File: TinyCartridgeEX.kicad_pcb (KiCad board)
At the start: 2 copper layers, 62 x 81.1 mm, 27 parts, among them J1 Conn_01x24, J2 Conn_01x24, U1 SN74LVC8T245, U2 SN74LVC8T245, U3 SN74LVC8T245, U4 74LV17A, U5 74LVC06A, U6 74LVC1G06, U7 74LVC2G132, U9 TinyFPGA_EX, X1 EXPANSION_PORT_C64_EDGE

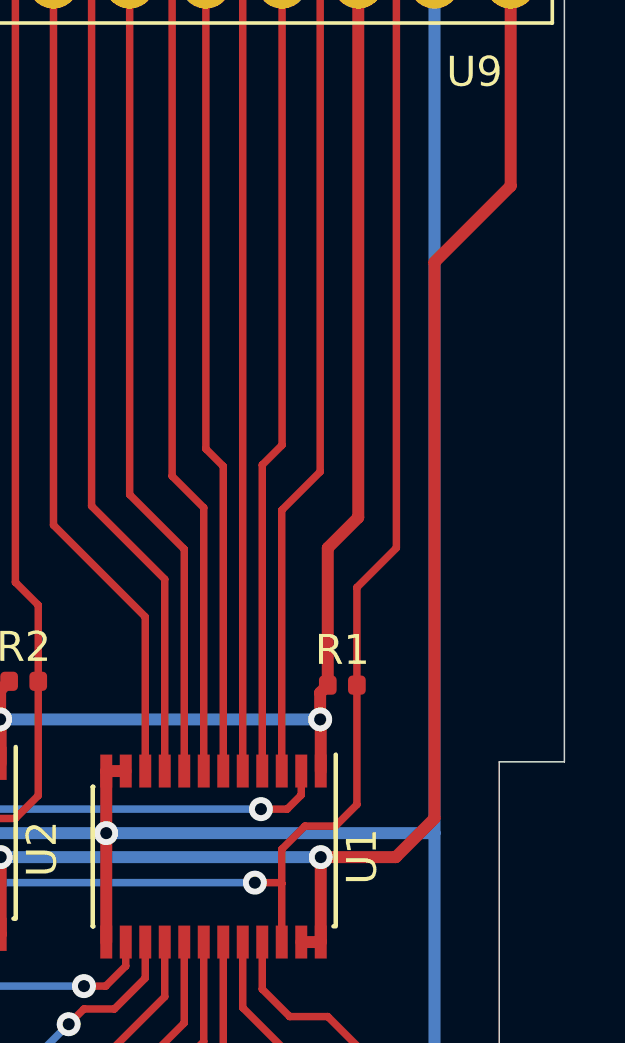
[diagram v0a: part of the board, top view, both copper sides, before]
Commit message: Add diode to Vin
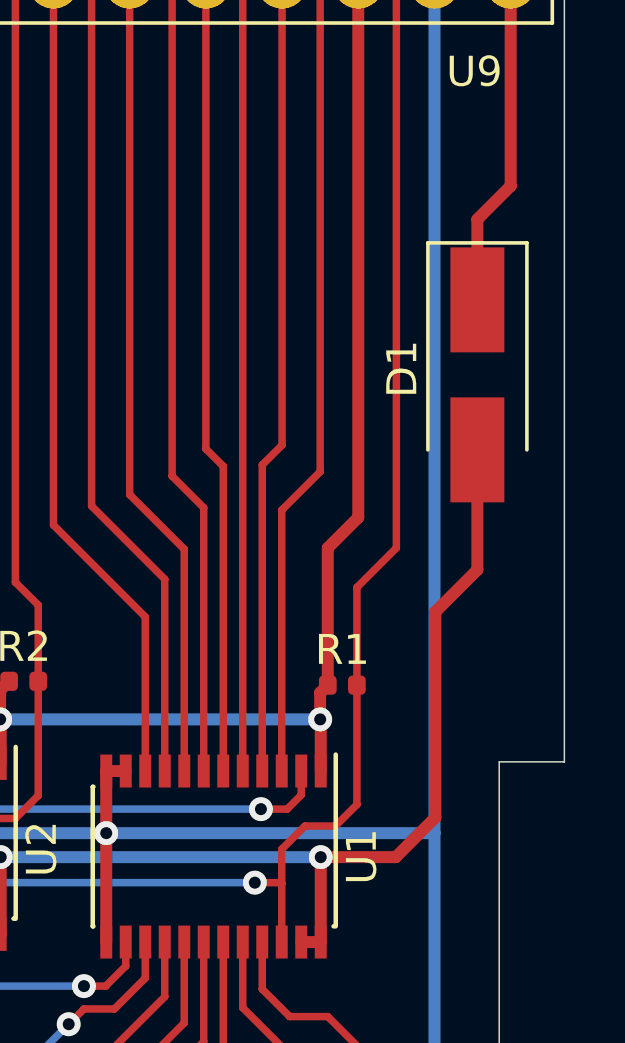
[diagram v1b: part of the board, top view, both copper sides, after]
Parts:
- added D1: EC30QSA045, Diode_SMD:D_SMA_Handsoldering, F.Cu at (104.3, 127.2)
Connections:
- U9 pad 48: +5V -> Net-(D1-Pad1)
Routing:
- net +5V: track 123.3 -> 107.2 mm
- net Net-(D1-Pad1): track 0.00 -> 11.0 mm
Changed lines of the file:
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@@
     (thickness 1.6)
     (drawings 20)
-    (tracks 723)
+    (tracks 726)
     (zones 0)
-    (modules 27)
-    (nets 85)
+    (modules 28)
+    (nets 86)
   )
   (page A4)
@@
   (net 83 "Net-(U7-Pad2)")
   (net 84 "Net-(U7-Pad1)")
+  (net 85 "Net-(D1-Pad1)")
   (net_class Default "This is the default net class."
     (clearance 0.2)
@@
     (add_net +5V)
     (add_net GND)
+    (add_net "Net-(D1-Pad1)")
     (add_net VCC)
+  )
+  (module Diode_SMD:D_SMA_Handsoldering (layer F.Cu)
+    (at 104.3 127.2 270)
+    (descr "Diode SMA (DO-214AC) Handsoldering")
+    (tags "Diode SMA (DO-214AC) Handsoldering")
+    (attr smd)
+    (fp_text reference D1 (at -0.2 2.5 90) (layer F.SilkS)
+      (effects (font (size 1 1) (thickness 0.15)))
+    )
+    (fp_text value EC30QSA045 (at 0 2.6 90) (layer F.Fab)
+      (effects (font (size 1 1) (thickness 0.15)))
+    )
+    (fp_line (start -4.4 -1.65) (end 2.5 -1.65) (layer F.SilkS) (width 0.12))
+    (fp_line (start -4.4 1.65) (end 2.5 1.65) (layer F.SilkS) (width 0.12))
+    (fp_line (start -0.64944 0.00102) (end 0.50118 -0.79908) (layer F.Fab) (width 0.1))
+    (fp_line (start -0.64944 0.00102) (end 0.50118 0.75032) (layer F.Fab) (width 0.1))
+    (fp_line (start 0.50118 0.75032) (end 0.50118 -0.79908) (layer F.Fab) (width 0.1))
+    (fp_line (start -0.64944 -0.79908) (end -0.64944 0.80112) (layer F.Fab) (width 0.1))
+    (fp_line (start 0.50118 0.00102) (end 1.4994 0.00102) (layer F.Fab) (width 0.1))
+    (fp_line (start -0.64944 0.00102) (end -1.55114 0.00102) (layer F.Fab) (width 0.1))
+    (fp_line (start -4.5 1.75) (end -4.5 -1.75) (layer F.CrtYd) (width 0.05))
+    (fp_line (start 4.5 1.75) (end -4.5 1.75) (layer F.CrtYd) (width 0.05))
+    (fp_line (start 4.5 -1.75) (end 4.5 1.75) (layer F.CrtYd) (width 0.05))
+    (fp_line (start -4.5 -1.75) (end 4.5 -1.75) (layer F.CrtYd) (width 0.05))
+    (fp_line (start 2.3 -1.5) (end -2.3 -1.5) (layer F.Fab) (width 0.1))
+    (fp_line (start 2.3 -1.5) (end 2.3 1.5) (layer F.Fab) (width 0.1))
+    (fp_line (start -2.3 1.5) (end -2.3 -1.5) (layer F.Fab) (width 0.1))
+    (fp_line (start 2.3 1.5) (end -2.3 1.5) (layer F.Fab) (width 0.1))
+    (fp_line (start -4.4 -1.65) (end -4.4 1.65) (layer F.SilkS) (width 0.12))
+    (fp_text user %R (at 0 -2.5 90) (layer F.Fab)
+      (effects (font (size 1 1) (thickness 0.15)))
+    )
+    (pad 2 smd rect (at 2.5 0 270) (size 3.5 1.8) (layers F.Cu F.Paste F.Mask)
+      (net 1 +5V))
+    (pad 1 smd rect (at -2.5 0 270) (size 3.5 1.8) (layers F.Cu F.Paste F.Mask)
+      (net 85 "Net-(D1-Pad1)"))
+    (model ${KISYS3DMOD}/Diode_SMD.3dshapes/D_SMA.wrl
+      (at (xyz 0 0 0))
+      (scale (xyz 1 1 1))
+      (rotate (xyz 0 0 0))
+    )
   )
   (module TinyFPGA:TinyFPGA_EX (layer F.Cu)
@@
     (fp_arc (start 7.62 -1.33) (end 6.62 -1.33) (angle -180) (layer F.SilkS) (width 0.12))
     (pad 48 thru_hole oval (at 15.24 0 270) (size 1.7 1.7) (drill 1) (layers *.Cu *.Mask)
-      (net 1 +5V))
+      (net 85 "Net-(D1-Pad1)"))
     (pad 24 thru_hole oval (at 0 58.42 270) (size 1.7 1.7) (drill 1) (layers *.Cu *.Mask)
       (net 65 GAME))
@@
   (segment (start 52.07 148.4885) (end 52.0955 148.463) (width 0.4) (layer F.Cu) (net 1))
   (segment (start 52.07 160.3248) (end 52.07 148.4885) (width 0.4) (layer F.Cu) (net 1))
-  (segment (start 102.87 141.986) (end 101.581 143.275) (width 0.4) (layer F.Cu) (net 1))
-  (segment (start 101.581 143.275) (end 99.079 143.275) (width 0.4) (layer F.Cu) (net 1))
-  (segment (start 102.87 123.444) (end 102.87 141.986) (width 0.4) (layer F.Cu) (net 1))
-  (segment (start 105.41 120.904) (end 102.87 123.444) (width 0.4) (layer F.Cu) (net 1))
-  (segment (start 105.41 120.904) (end 105.41 114.141) (width 0.4) (layer F.Cu) (net 1))
+  (segment (start 105.41 120.904) (end 105.41 114.141) (width 0.4) (layer F.Cu) (net 85))
+  (segment (start 104.3 124.7) (end 104.3 122.014) (width 0.4) (layer F.Cu) (net 85))
+  (segment (start 104.3 122.014) (end 105.41 120.904) (width 0.4) (layer F.Cu) (net 85))
   (segment (start 52.0955 147.4725) (end 52.0955 148.463) (width 0.4) (layer F.Cu) (net 1))
   (segment (start 49.53 144.907) (end 52.0955 147.4725) (width 0.4) (layer F.Cu) (net 1))
@@
   (segment (start 55.245 136.017) (end 57.023 137.795) (width 0.4) (layer B.Cu) (net 1))
   (segment (start 52.07 156.3248) (end 54.61 156.3248) (width 0.4) (layer F.Cu) (net 1))
+  (segment (start 102.9 141.956) (end 101.581 143.275) (width 0.4) (layer F.Cu) (net 1))
+  (segment (start 101.581 143.275) (end 99.079 143.275) (width 0.4) (layer F.Cu) (net 1))
+  (segment (start 102.9 135.1) (end 102.9 141.956) (width 0.4) (layer F.Cu) (net 1))
+  (segment (start 104.3 129.7) (end 104.3 133.7) (width 0.4) (layer F.Cu) (net 1))
+  (segment (start 104.3 133.7) (end 102.9 135.1) (width 0.4) (layer F.Cu) (net 1))
   (segment (start 91.929 140.406) (end 92.579 140.406) (width 0.4) (layer F.Cu) (net 2))
   (segment (start 81.261 142.475) (end 81.261 145.852) (width 0.4) (layer F.Cu) (net 2))
